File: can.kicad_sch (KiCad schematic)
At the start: 2 parts, among them U2 ISO1042-Q1

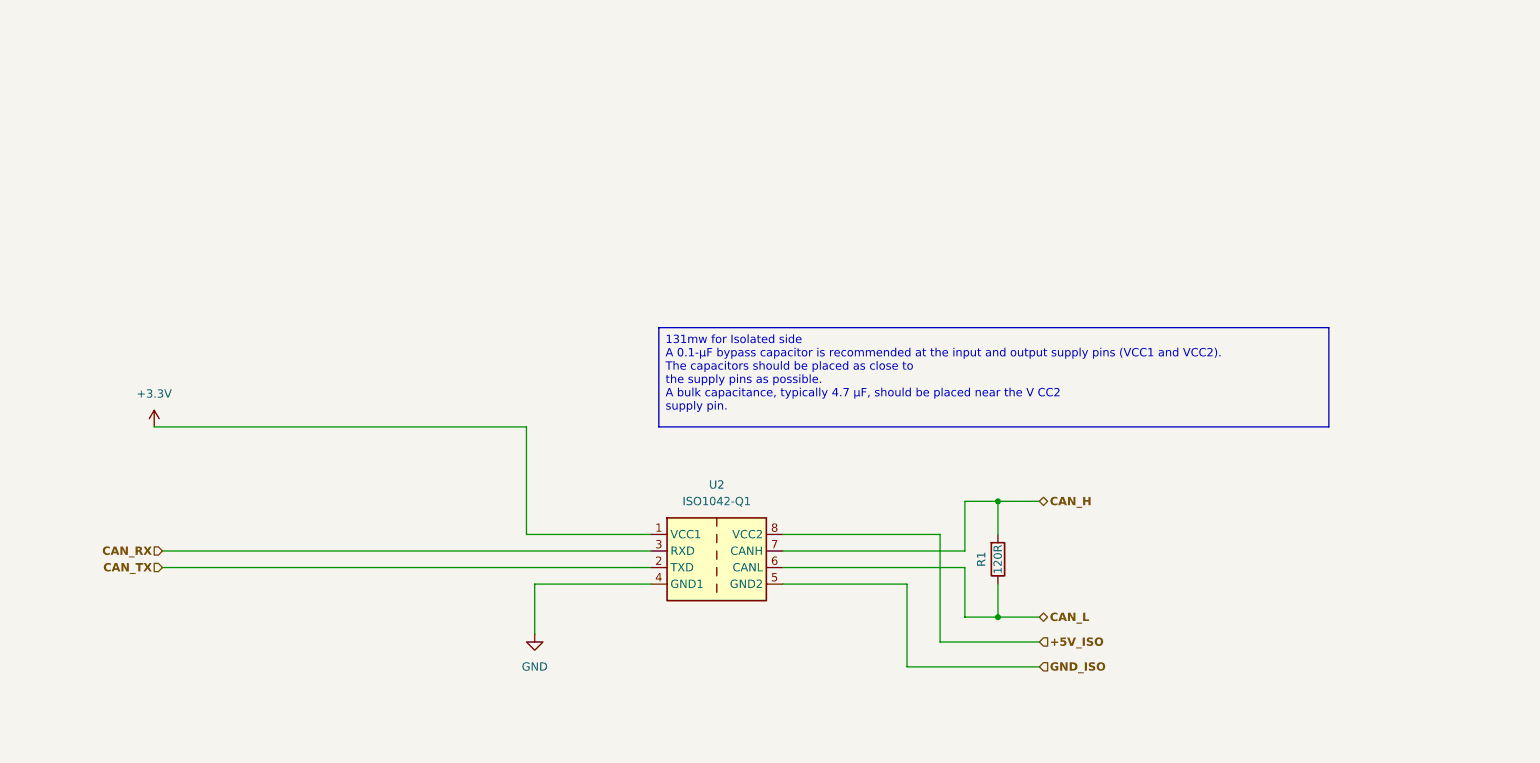
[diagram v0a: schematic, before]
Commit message: version 2 initial
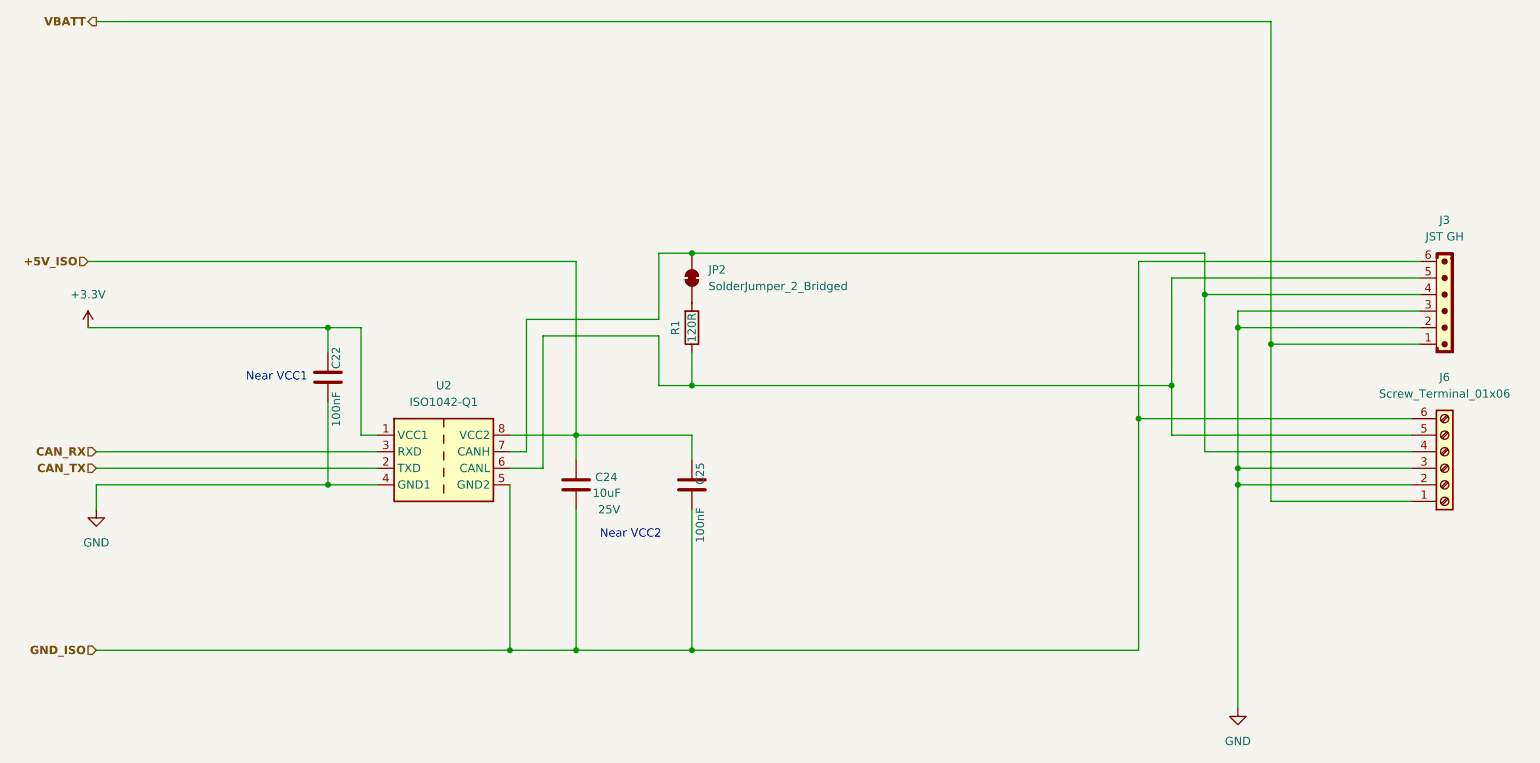
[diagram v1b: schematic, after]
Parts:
- added C22, C25: 100nF, Capacitor_SMD:C_0603_1608Metric, symbol Device:C
- added C24: 10uF, Capacitor_SMD:C_0805_2012Metric, symbol Device:C
- added J3: JST GH, dnt:JST_GH_BM06B-GHS-TBT_1x06-1MP_P1.25mm_Vertical, symbol PCM_SL_Connectors:JST_06
- added J6: Screw_Terminal_01x06, TerminalBlock_Phoenix:TerminalBlock_Phoenix_PT-1,5-6-3.5-H_1x06_P3.50mm_Horizontal, symbol Connector:Screw_Terminal_01x06
- added JP2: SolderJumper_2_Bridged, Jumper:SolderJumper-2_P1.3mm_Open_TrianglePad1.0x1.5mm, symbol Jumper:SolderJumper_2_Bridged
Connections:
- net +3.3V: now also C22.1
- net +5V_ISO: now also C24.1, C25.1
- net GND: now also C22.2, J3.2, J3.3, J6.2 (Pin_2), J6.3 (Pin_3)
- net GND_ISO: now also C24.2, C25.2, J3.6, J6.6 (Pin_6)
- net CAN_H: no longer names the net of R1.2
- net CAN_H: now also JP2.1 (A); no longer U2.7 (CANH)
- net CAN_L: no longer names the net of R1.1, U2.6 (CANL)
- net CAN_L: now also J3.5, J6.5 (Pin_5)
- new net: J3.4, J6.4 (Pin_4), JP2.2 (B), U2.7 (CANH)
- new net VBATT: J3.1, J6.1 (Pin_1)
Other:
- note added: "Near VCC1"
- note added: "Near VCC2"
- moved on the sheet: R1, U2
